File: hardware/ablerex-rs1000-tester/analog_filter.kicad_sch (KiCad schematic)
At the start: 148 parts, among them U16 TL074, U17 TL072, U18 TL074, U19 TL074, U20 TL074, U9 LM339

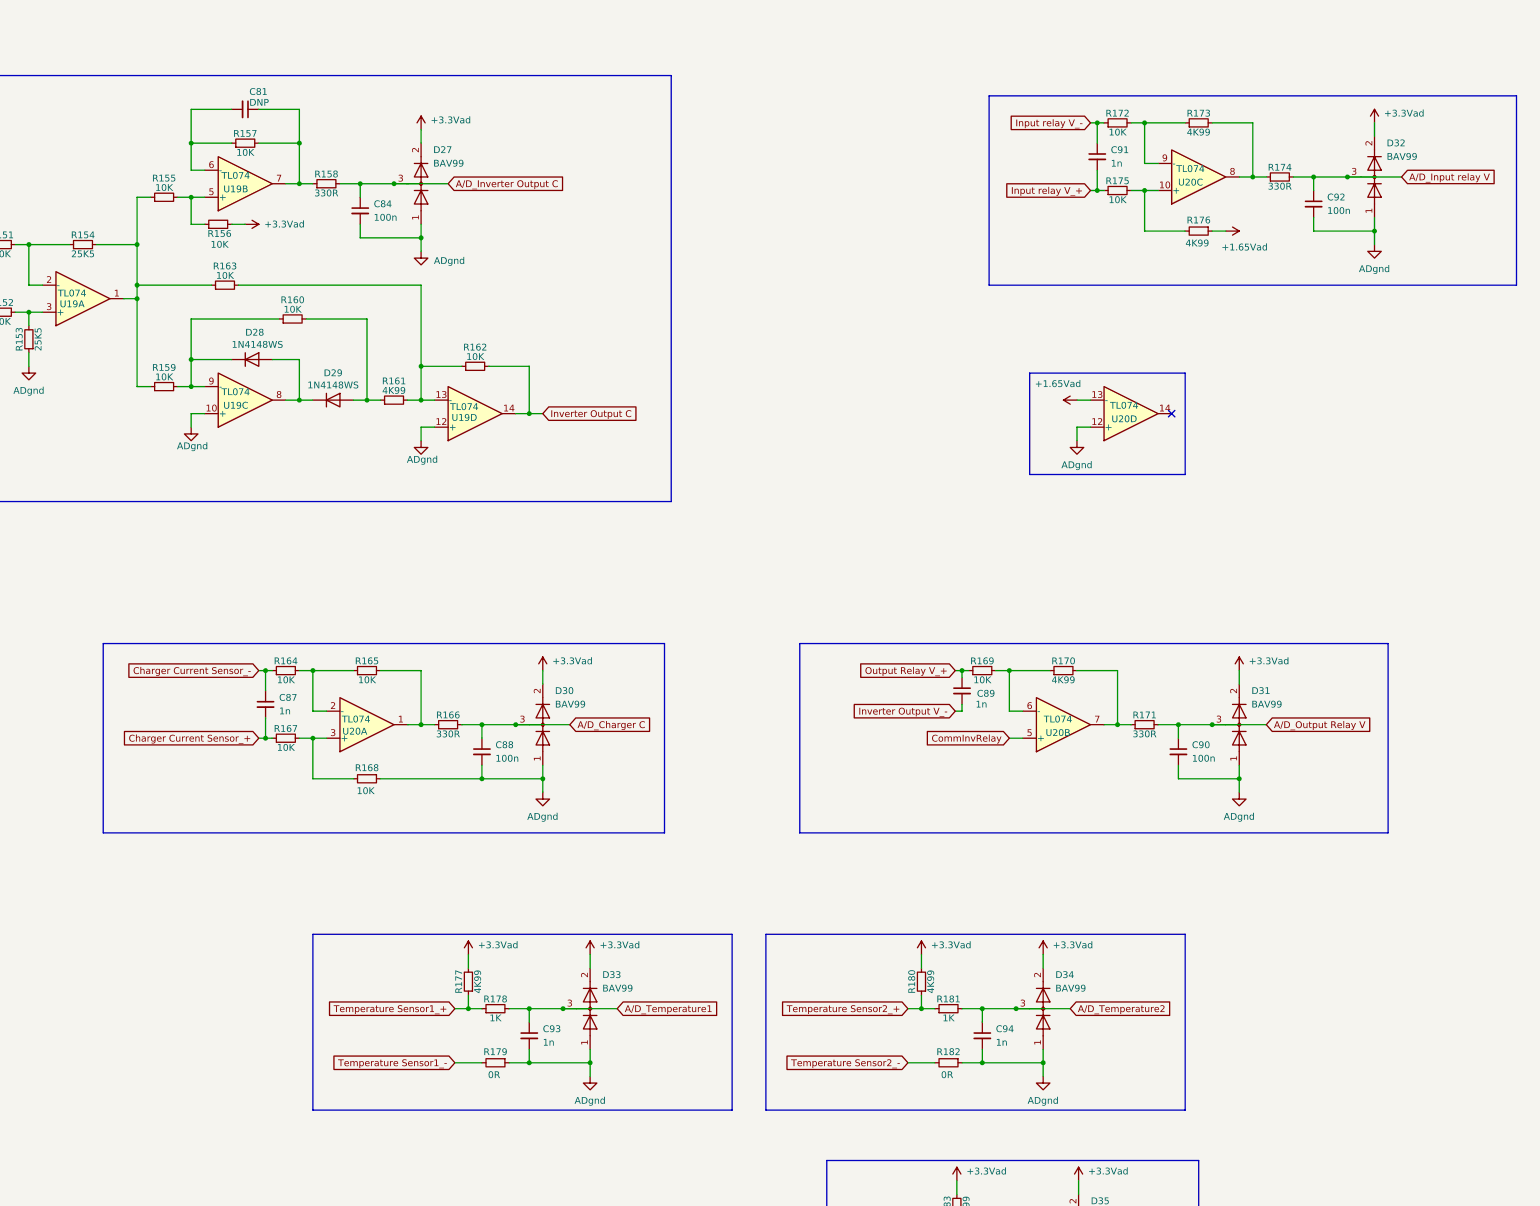
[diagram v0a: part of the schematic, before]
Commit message: checked all the schematics
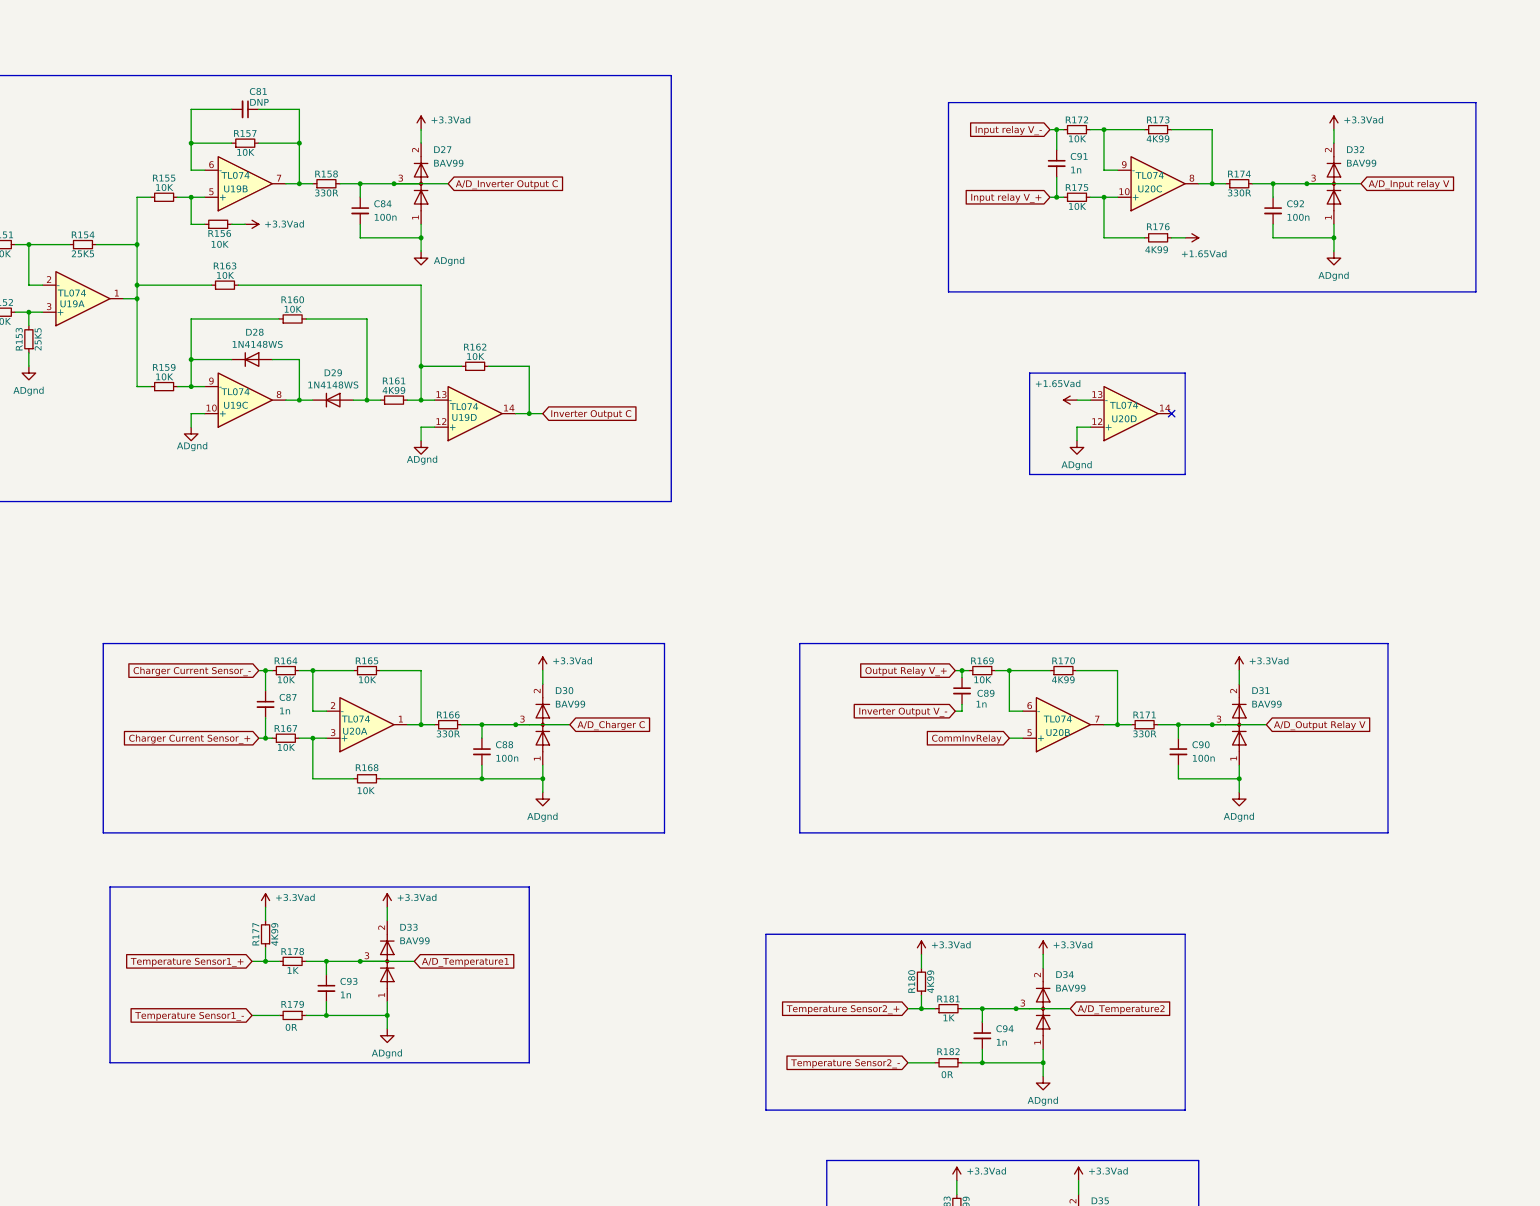
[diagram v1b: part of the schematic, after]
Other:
- moved on the sheet: C91, C92, C93, D32, D33, R172, R173, R174, R175, R176, R177, R178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
